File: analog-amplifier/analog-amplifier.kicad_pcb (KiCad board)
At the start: 2 copper layers, 58.5 x 42 mm, 48 parts, among them J1 Conn_Coaxial_Small, J2 Conn_Coaxial_Small, J3 Conn_Coaxial_Small, J4 Conn_Coaxial_Small, J5 Conn_01x01_Socket, J6 Conn_01x01_Socket, U1 LT6202, U2 LT6404IUD, U3 LT6202, U4 LT6404IUD

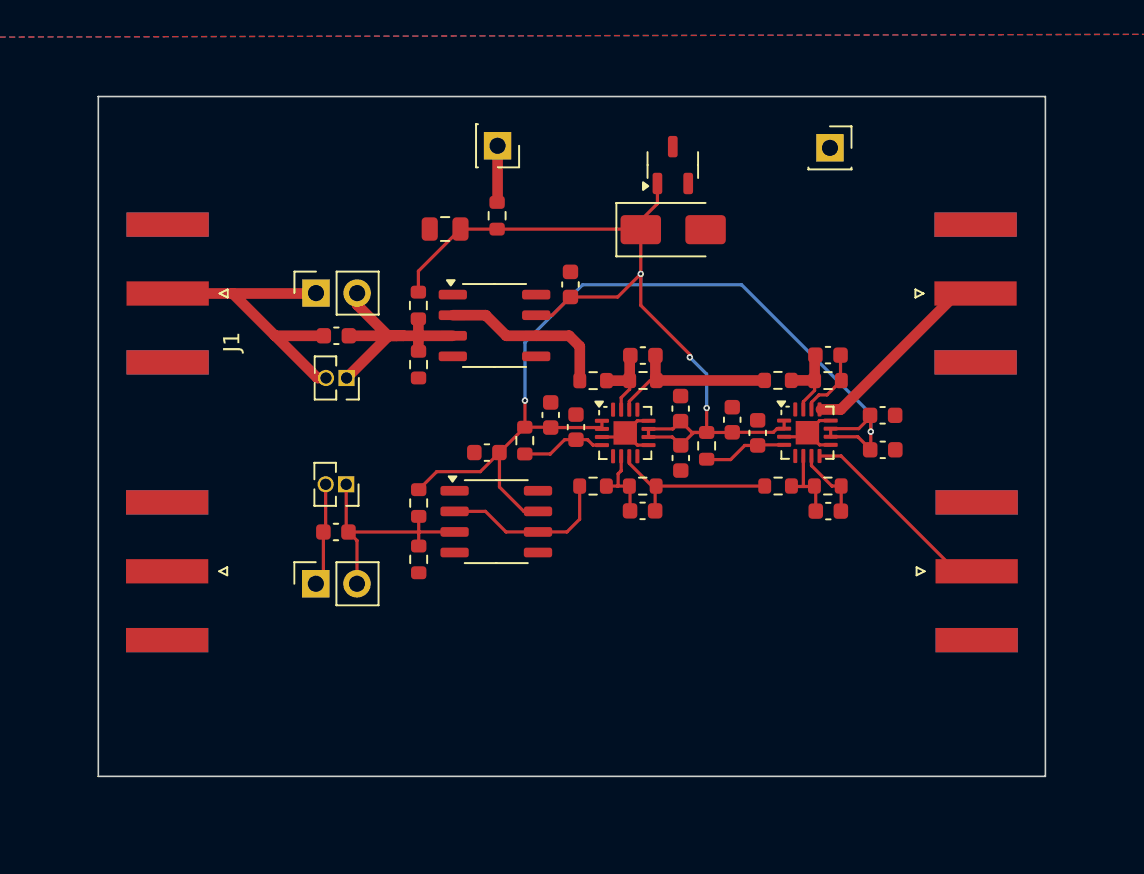
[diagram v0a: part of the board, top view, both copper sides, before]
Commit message: Finished Beta
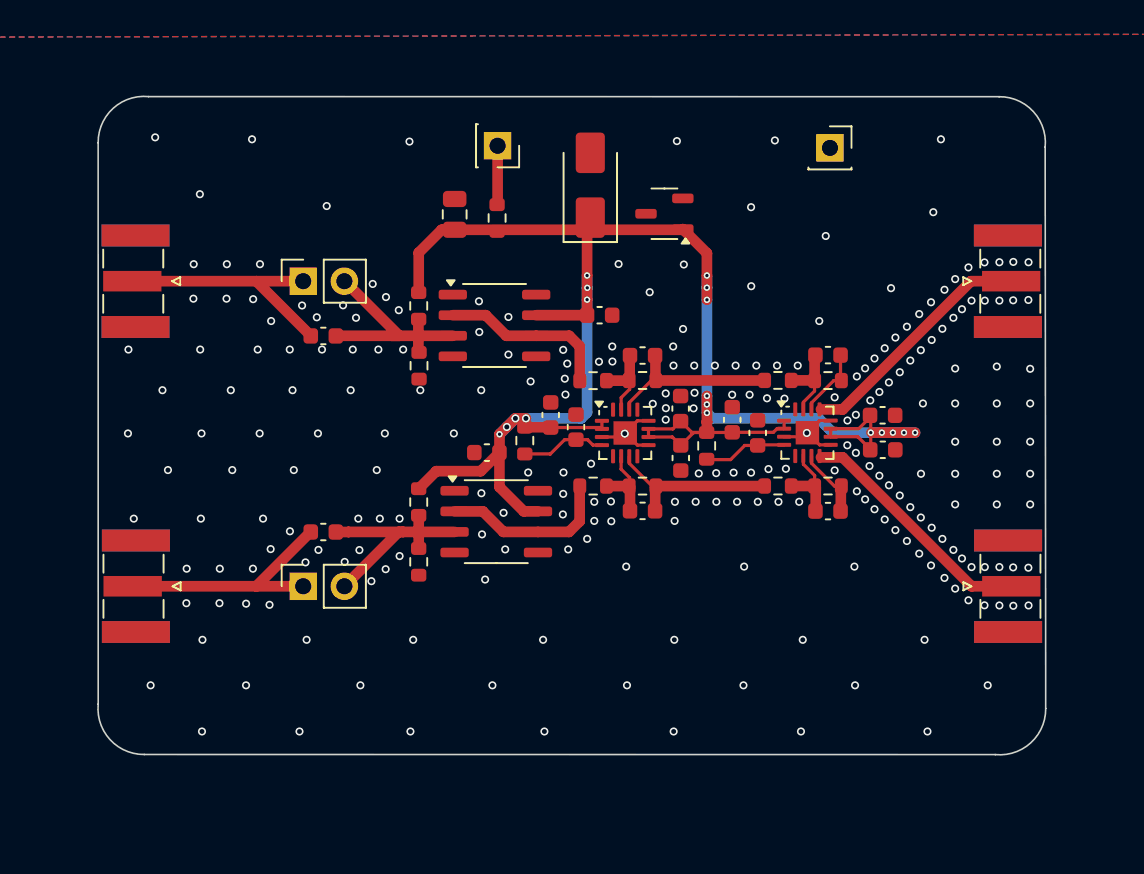
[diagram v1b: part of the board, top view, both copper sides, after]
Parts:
- removed JP3, JP4: Jumper_2_Open, Connector_PinSocket_1.27mm:PinSocket_1x02_P1.27mm_Vertical
- J1, J2, J3, J4: footprint Connector_Coaxial:SMA_Amphenol_132289_EdgeMount -> Connector_Coaxial:SMA_Samtec_SMA-J-P-X-ST-EM1_EdgeMount
- moved D2 5.81 mm to (126.8, 73.1), turned to 90 degrees
- moved D1 3.05 mm to (131.3, 74.8), turned to 180 degrees
- moved C13 2.62 mm to (127.3, 81.1), turned to 0 degrees
- moved J4 2.15 mm to (152.6, 97.8), turned to 90 degrees
- moved J2 2.14 mm to (98.7, 97.8), turned to -90 degrees
- moved J3 2.14 mm to (152.6, 79.0), turned to 90 degrees
- moved J1 2.12 mm to (98.7, 79.0), turned to -90 degrees
- moved C8 1.08 mm to (118.4, 74.9), turned to 90 degrees
- moved JP1 1.08 mm to (109.0, 79.0)
- moved C2 0.81 mm to (110.3, 82.4)
- moved JP2 0.80 mm to (109.0, 97.8)
- moved C5 0.78 mm to (110.3, 94.5)
- moved R9 0.15 mm to (116.2, 96.3)
- moved F1 0.14 mm to (121.0, 75.1)
- moved R4 0.08 mm to (116.2, 84.2)
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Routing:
- net /IN-: track 6.43 -> 15.5 mm
- net /IN+: track 20.1 -> 15.5 mm
- net Net-(JP1-B): track 17.5 -> 14.4 mm
- net /OUT-: track 12.5 -> 15.3 mm
- net /OUT+: track 12.6 -> 15.3 mm
- net +5V: track 113.7 -> 115.2 mm, vias 5 -> 18
- net Net-(JP2-B): track 14.9 -> 14.1 mm
- net GND: vias 0 -> 248
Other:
- board size 58.5 x 42 mm -> 58.5 x 40.6 mm
- board text added: "{ "ViaStitching": "0.2", "stitch_zone_0": { "HSpacing": "1", "VSpacing": "1", "Clearance": "0", "Randomize": false }, "stitch_zone_1": { "HSpacing": "2", "VSpacing": "2", "Clearance": "5", "Randomize": false }, "stitch_zone_2": { "HSpacing": "1", "VSpacing": "1", "Clearance": "0.2", "Randomize": false } }"
